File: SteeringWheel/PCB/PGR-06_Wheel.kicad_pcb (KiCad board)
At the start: 2 copper layers, 85.1 x 104.1 mm, 61 parts, among them J14 SWD, SW1 SW_SPDT, U3 LM2575HVS-3.3_NOPB, U6 STM32F405RGT6, Y1 16MHz

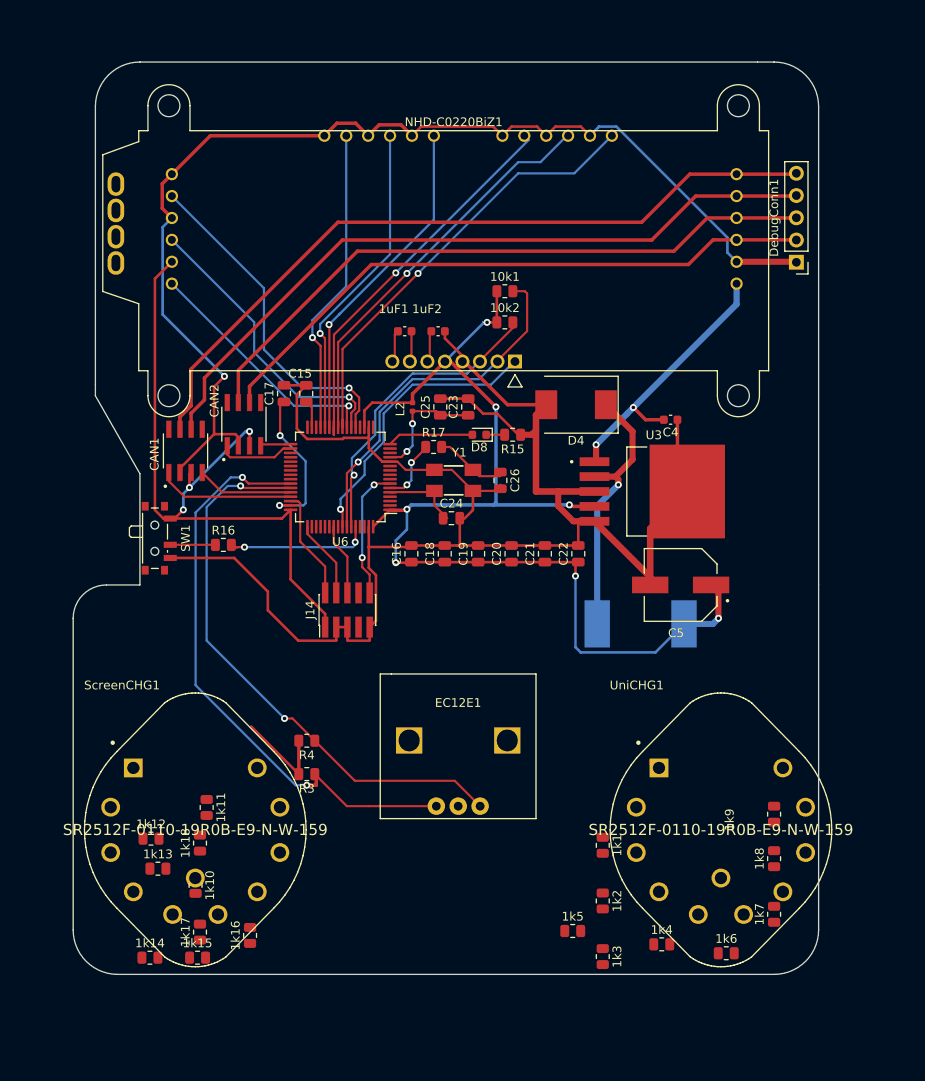
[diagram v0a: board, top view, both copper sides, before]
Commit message: Steering Wheel Update
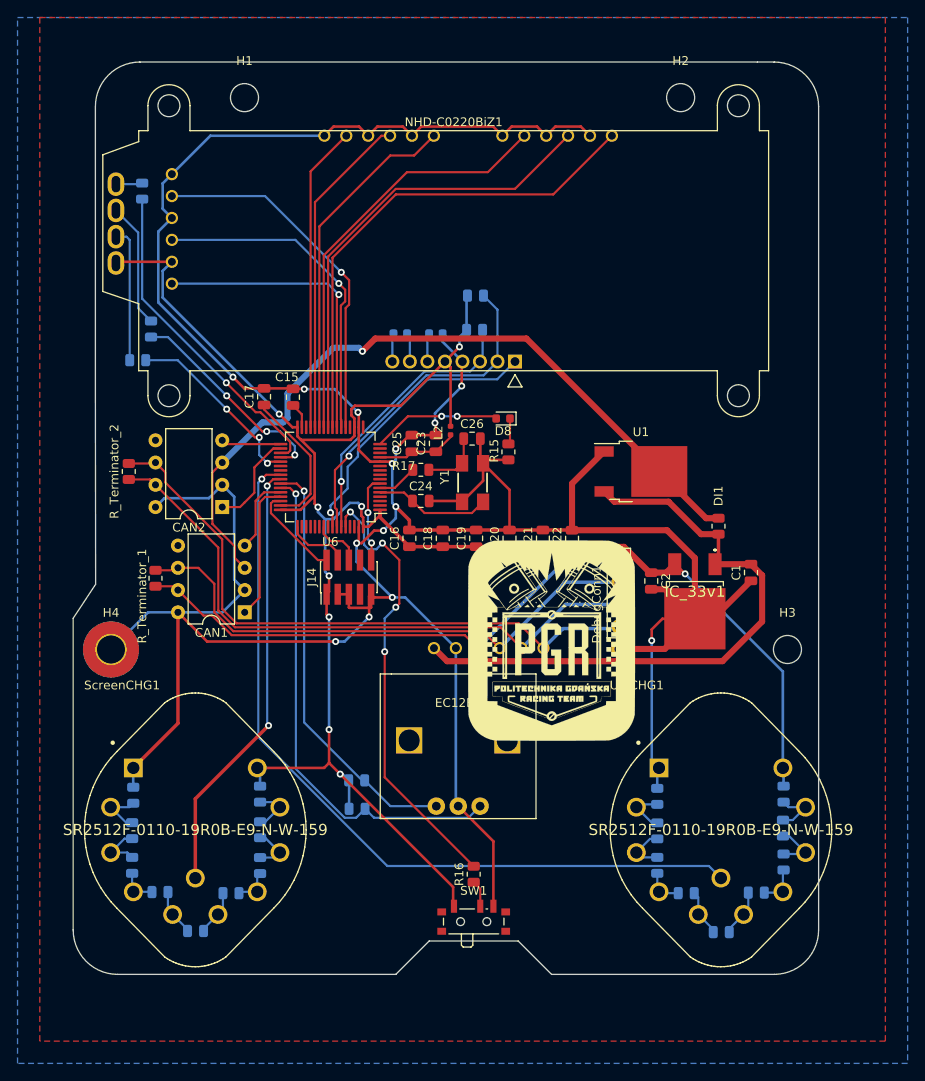
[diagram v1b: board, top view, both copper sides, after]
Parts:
- removed C4: 100uF, Capacitor_SMD:C_0603_1608Metric
- removed C5: 16SVPG330MX, 16SVPG330MX:CAP_16SVPG330MX
- removed D4: 1N5819, Diode_SMD:D_SMC
- removed L3.3: 330uH, PGR-06_Additional:7447707331
- removed U3: LM2575HVS-3.3_NOPB, LM2575HVS-3.3_NOPB:VREG_TPS79625KTTR
- added C1: BD_CAP2, Capacitor_SMD:C_0805_2012Metric, F.Cu at (147.2, 126.8)
- added C2: BD_CAP1, Capacitor_SMD:C_0805_2012Metric, F.Cu at (135.8, 127.8)
- added DI1: 0Ohm, Resistor_SMD:R_0805_2012Metric, F.Cu at (143.5, 121.6)
- added G***: LOGO, PGR-06_Additional:logo, B.Cu at (142.2, 83.8)
- added G***: LOGO, PGR-06_Additional:logo, F.Cu at (124.5, 134.6)
- added H1: MountingHole, MountingHole:MountingHole_3.2mm_M3, F.Cu at (89.4, 72.6)
- added H2: MountingHole, MountingHole:MountingHole_3.2mm_M3, F.Cu at (139.2, 72.6)
- added H3: MountingHole, MountingHole:MountingHole_3.2mm_M3, F.Cu at (151.4, 135.6)
- added H4: MountingHole_Pad, MountingHole:MountingHole_3.2mm_M3_Pad_TopBottom, F.Cu at (74.2, 135.6)
- added IC_33v1: BD733L5FP-CE2, PGR-06_Additional:BD750L5FPCE2, F.Cu at (140.8, 133.9)
- added LED_B1: R_Small, Resistor_SMD:R_0805_2012Metric, B.Cu at (77.7, 83.3)
- added LED_G1: R_Small, Resistor_SMD:R_0805_2012Metric, B.Cu at (78.7, 99.1)
- added LED_R1: R_Small, Resistor_SMD:R_0805_2012Metric, B.Cu at (77.2, 102.6)
- added R_Terminator_1: 120Ohm, Resistor_SMD:R_0805_2012Metric, F.Cu at (79.2, 127.5)
- added R_Terminator_2: 120Ohm, Resistor_SMD:R_0805_2012Metric, F.Cu at (76.2, 115.3)
- added U1: LM1117-5.0, Package_TO_SOT_SMD:TO-252-2, F.Cu at (134.7, 115.3)
- 10k1, 10k2, 1k1, 1k10, 1k11, 1k12, 1k13, 1k14, 1k15, 1k16, 1k17, 1k18, 1k2, 1k3, 1k4, 1k5, 1k6, 1k7, 1k8, 1k9, 1uF1, 1uF2, R3, R4: moved to B.Cu
- CAN1, CAN2: value SN65HVD230MDREP -> MCP2561-E-P; footprint PGR-06_Additional:SOIC127P599X175-8N -> Package_DIP:DIP-8_W7.62mm
- moved SW1 56.5 mm to (115.6, 166.4), turned to 0 degrees
- moved MAIN1 51.9 mm to (117.3, 132.8), turned to 180 degrees
- moved DebugConn1 48.6 mm to (132.1, 135.6)
- moved R16 47.2 mm to (115.6, 161.3), turned to 90 degrees
- moved CAN1 19.6 mm to (89.4, 131.4), turned to 180 degrees
- moved 1k5 17.0 mm to (143.8, 167.9)
- moved 1k17 13.5 mm to (91.2, 156.2)
- moved 1k10 12.5 mm to (76.7, 152.3)
- moved 1k3 12.1 mm to (136.5, 160.3)
- moved 1k2 10.1 mm to (136.5, 156.3)
- moved CAN2 9.78 mm to (86.9, 119.4), turned to 180 degrees
- moved R4 9.66 mm to (102.3, 153.8)
- moved 1k11 8.91 mm to (76.6, 156.3)
- moved 1k18 8.85 mm to (91.2, 152.1)
- moved 1k1 8.36 mm to (136.5, 152.4)
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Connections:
- CAN1 pad 3: +3V3 -> +5V
- CAN1 pad 8: (no net) -> GND
- CAN2 pad 3: +3V3 -> +5V
- CAN2 pad 8: (no net) -> GND
- MAIN1 pad 1: CAN1_H -> CAN2_L
- MAIN1 pad 2: CAN1_L -> CAN2_H
- MAIN1 pad 3: CAN2_H -> CAN1_L
- MAIN1 pad 4: CAN2_L -> CAN1_H
- MAIN1 pad 6: +12V -> VDD
- NHD-C0220BiZ1 pad 10: (no net) -> Net-(LED_R1-Pad2)
- NHD-C0220BiZ1 pad 11: (no net) -> Net-(LED_G1-Pad2)
- NHD-C0220BiZ1 pad 12: (no net) -> Net-(LED_B1-Pad2)
- U6 pad 15: /Rotaries/ROT_SCR -> (no net)
- U6 pad 35: (no net) -> /STM32F405RGT6/LED_B
- U6 pad 36: (no net) -> /STM32F405RGT6/LED_G
- U6 pad 37: (no net) -> /STM32F405RGT6/LED_R
- U6 pad 40: (no net) -> /Rotaries/ROT_UNI
- U6 pad 41: (no net) -> /Rotaries/ROT_SCR
- UniCHG1 pad 11: /Rotaries/ROT_SCR -> /Rotaries/ROT_UNI
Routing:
- net /Rotaries/ROT_UNI: track 0.00 -> 91.4 mm, vias 0 -> 1
- net GND: track 328.4 -> 416.3 mm, vias 1 -> 14
- net +5V: track 0.00 -> 87.0 mm, vias 0 -> 1
- net VDD: track 0.00 -> 69.8 mm
- net /Rotaries/ROT_SCR: track 0.00 -> 50.2 mm, vias 0 -> 2
- net /STM32F405RGT6/LED_B: track 0.00 -> 37.2 mm, vias 0 -> 1
- net BOOT0: track 18.2 -> 51.5 mm, vias 2 -> 4
- net +12V: track 31.1 -> 0.00 mm, vias 2 -> 0
- net Net-(D4-Pad1): track 30.6 -> 0.00 mm, vias 1 -> 0
- net CAN1_H: track 85.7 -> 60.0 mm
- net /STM32F405RGT6/LED_G: track 0.00 -> 24.3 mm, vias 0 -> 3
- net /STM32F405RGT6/LED_R: track 0.00 -> 21.5 mm, vias 0 -> 3
- net CAN1_L: track 82.7 -> 61.8 mm
- net /Rotaries/ENC_A: track 68.2 -> 48.5 mm, vias 2 -> 1
- net Net-(LED_R1-Pad2): track 0.00 -> 15.5 mm
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- added copper zone on B.Cu, net +3V3
- added copper zone on F.Cu, net GND
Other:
- outline, holes or cut-outs redrawn
